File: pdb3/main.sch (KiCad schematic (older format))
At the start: 5 parts, among them U1 AUIPS7111S

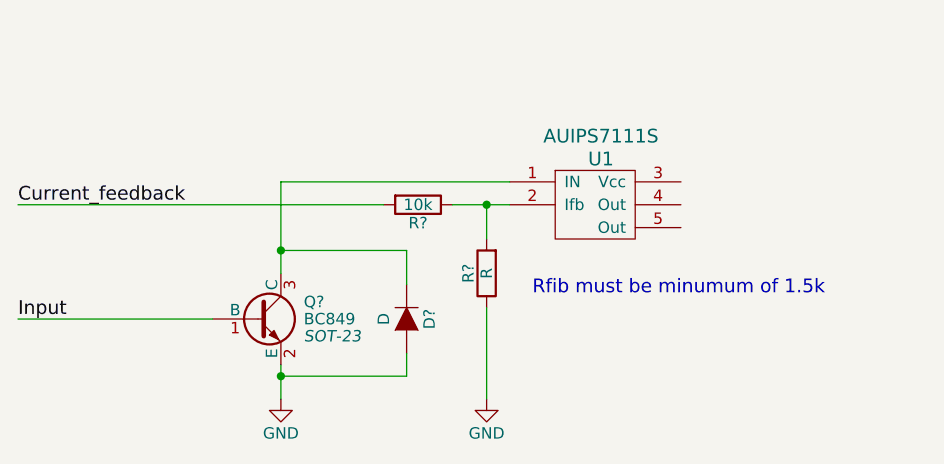
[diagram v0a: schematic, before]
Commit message: test
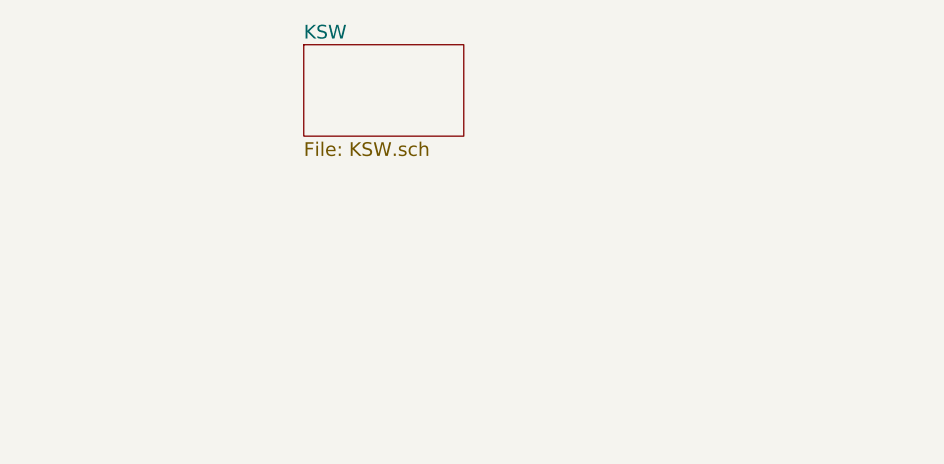
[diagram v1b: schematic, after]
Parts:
- removed D?: D, symbol D
- removed Q?: BC849, SOT-23, symbol BC849
- removed R?: 10k, symbol R
- removed R?: R, symbol R
- removed U1: AUIPS7111S, TO_SOT_Packages_SMD:TO-263-5Lead, symbol AUIPS7111S
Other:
- note removed: "Rfib must be minumum of 1.5k"
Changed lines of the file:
@@
 LIBS:dev_ic
 LIBS:dev_conn
+LIBS:main-cache
 EELAYER 25 0
 EELAYER END
 $Descr A4 11693 8268
 encoding utf-8
-Sheet 1 1
+Sheet 1 2
 Title ""
 Date ""
@@
 Comment4 ""
 $EndDescr
-$Comp
-L AUIPS7111S U1
-U 1 1 582DE54E
-P 4450 3400
-F 0 "U1" H 4450 3650 60  0000 C CNN
-F 1 "AUIPS7111S" H 4450 3750 60  0000 C CNN
-F 2 "TO_SOT_Packages_SMD:TO-263-5Lead" H 4450 3400 60  0001 C CNN
-F 3 "http://www.farnell.com/datasheets/1441780.pdf" H 4600 4000 60  0001 C CNN
-	1    4450 3400
-	1    0    0    -1
-$EndComp
-$Comp
-L R R?
-U 1 1 582DE7F7
-P 3650 3350
-F 0 "R?" V 3730 3350 50  0000 C CNN
-F 1 "10k" V 3650 3350 50  0000 C CNN
-F 2 "" V 3580 3350 50  0000 C CNN
-F 3 "" H 3650 3350 50  0000 C CNN
-	1    3650 3350
-	0    1    1    0
-$EndComp
-$Comp
-L R R?
-U 1 1 582DE84C
-P 3950 3650
-F 0 "R?" V 4030 3650 50  0000 C CNN
-F 1 "R" V 3950 3650 50  0000 C CNN
-F 2 "" V 3880 3650 50  0000 C CNN
-F 3 "" H 3950 3650 50  0000 C CNN
-	1    3950 3650
-	-1   0    0    1
-$EndComp
-Wire Wire Line
-	3950 3500 3950 3350
-Wire Wire Line
-	3800 3350 4050 3350
-Connection ~ 3950 3350
-Text Notes 4150 3750 0    60   ~ 0
-Rfib must be minumum of 1.5k
-$Comp
-L BC849 Q?
-U 1 1 582DE9C1
-P 2950 3850
-F 0 "Q?" H 3150 3925 50  0000 L CNN
-F 1 "BC849" H 3150 3850 50  0000 L CNN
-F 2 "SOT-23" H 3150 3775 50  0000 L CIN
-F 3 "" H 2950 3850 50  0000 L CNN
-	1    2950 3850
-	1    0    0    -1
-$EndComp
-Wire Wire Line
-	4050 3250 3050 3250
-Wire Wire Line
-	3050 3250 3050 3650
-Wire Wire Line
-	1900 3850 2750 3850
-Wire Wire Line
-	3050 4050 3050 4200
-$Comp
-L GND #PWR?
-U 1 1 582DEB23
-P 3050 4200
-F 0 "#PWR?" H 3050 3950 50  0001 C CNN
-F 1 "GND" H 3050 4050 50  0000 C CNN
-F 2 "" H 3050 4200 50  0000 C CNN
-F 3 "" H 3050 4200 50  0000 C CNN
-	1    3050 4200
-	1    0    0    -1
-$EndComp
-$Comp
-L GND #PWR?
-U 1 1 582DEB41
-P 3950 4200
-F 0 "#PWR?" H 3950 3950 50  0001 C CNN
-F 1 "GND" H 3950 4050 50  0000 C CNN
-F 2 "" H 3950 4200 50  0000 C CNN
-F 3 "" H 3950 4200 50  0000 C CNN
-	1    3950 4200
-	1    0    0    -1
-$EndComp
-Wire Wire Line
-	3950 3800 3950 4200
-Wire Wire Line
-	3500 3350 1900 3350
-Text Label 1900 3850 0    60   ~ 0
-Input
-Text Label 1900 3350 0    60   ~ 0
-Current_feedback
-$Comp
-L D D?
-U 1 1 582DEC68
-P 3600 3850
-F 0 "D?" H 3600 3950 50  0000 C CNN
-F 1 "D" H 3600 3750 50  0000 C CNN
-F 2 "" H 3600 3850 50  0000 C CNN
-F 3 "" H 3600 3850 50  0000 C CNN
-	1    3600 3850
-	0    1    1    0
-$EndComp
-Wire Wire Line
-	3600 4000 3600 4100
-Wire Wire Line
-	3600 4100 3050 4100
-Connection ~ 3050 4100
-Wire Wire Line
-	3600 3700 3600 3550
-Wire Wire Line
-	3600 3550 3050 3550
-Connection ~ 3050 3550
+$Sheet
+S 3150 2650 700  400
+U 582DFA3C
+F0 "KSW" 60
+F1 "KSW.sch" 60
+$EndSheet
 $EndSCHEMATC
